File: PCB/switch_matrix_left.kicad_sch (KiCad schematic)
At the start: 80 parts, among them SW1 SW_Push, SW10 SW_Push, SW11 SW_Push, SW12 SW_Push, SW13 SW_Push, SW14 SW_Push, SW15 SW_Push, SW16 SW_Push, SW17 SW_Push, SW18 SW_Push, SW19 SW_Push, SW2 SW_Push, SW20 SW_Push, SW21 SW_Push, SW22 SW_Push, SW23 SW_Push, SW24 SW_Push, SW25 SW_Push, SW26 SW_Push, SW27 SW_Push, SW28 SW_Push, SW29 SW_Push, SW3 SW_Push, SW30 SW_Push, SW31 SW_Push, SW32 SW_Push, SW33 SW_Push, SW34 SW_Push, SW35 SW_Push, SW36 SW_Push, SW37 SW_Push, SW38 SW_Push, SW39 SW_Push, SW4 SW_Push, SW40 RotaryEncoder_Switch, SW5 SW_Push, SW6 SW_Push, SW7 SW_Push, SW8 SW_Push, SW9 SW_Push

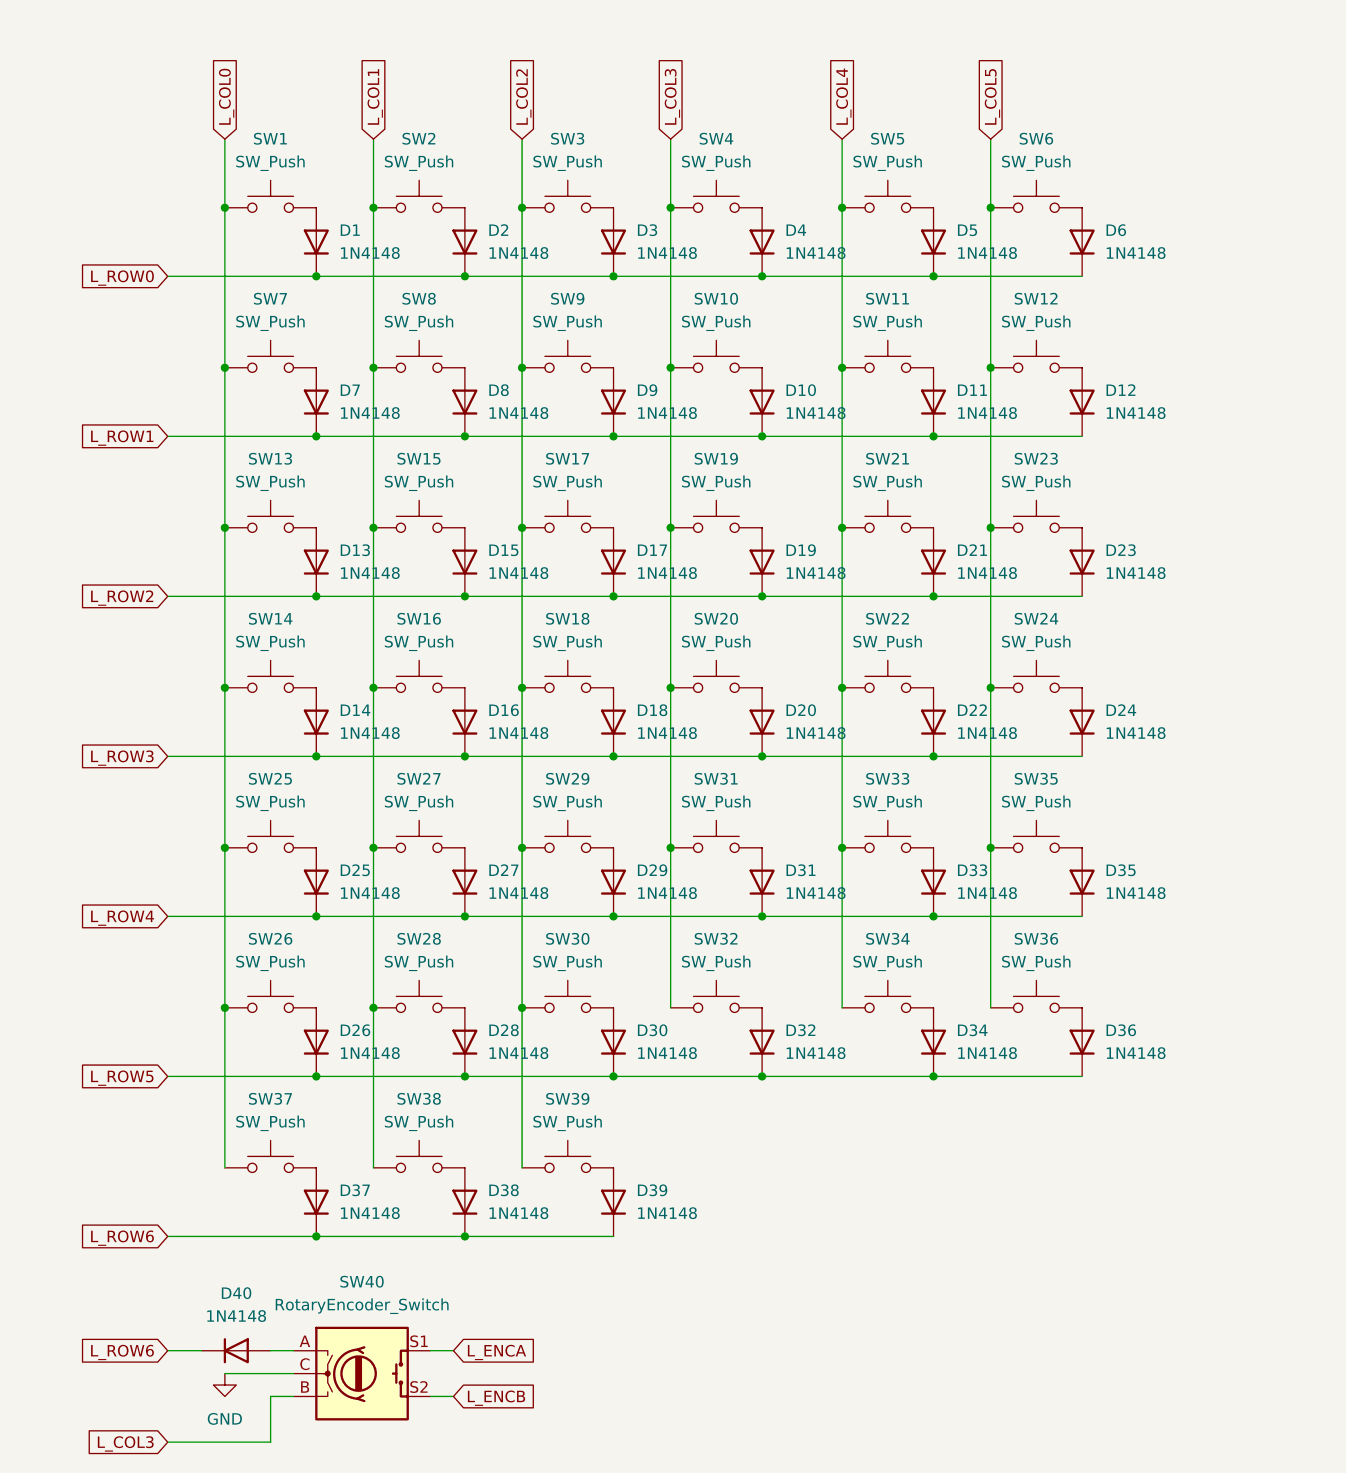
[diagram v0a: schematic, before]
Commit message: updated schematic
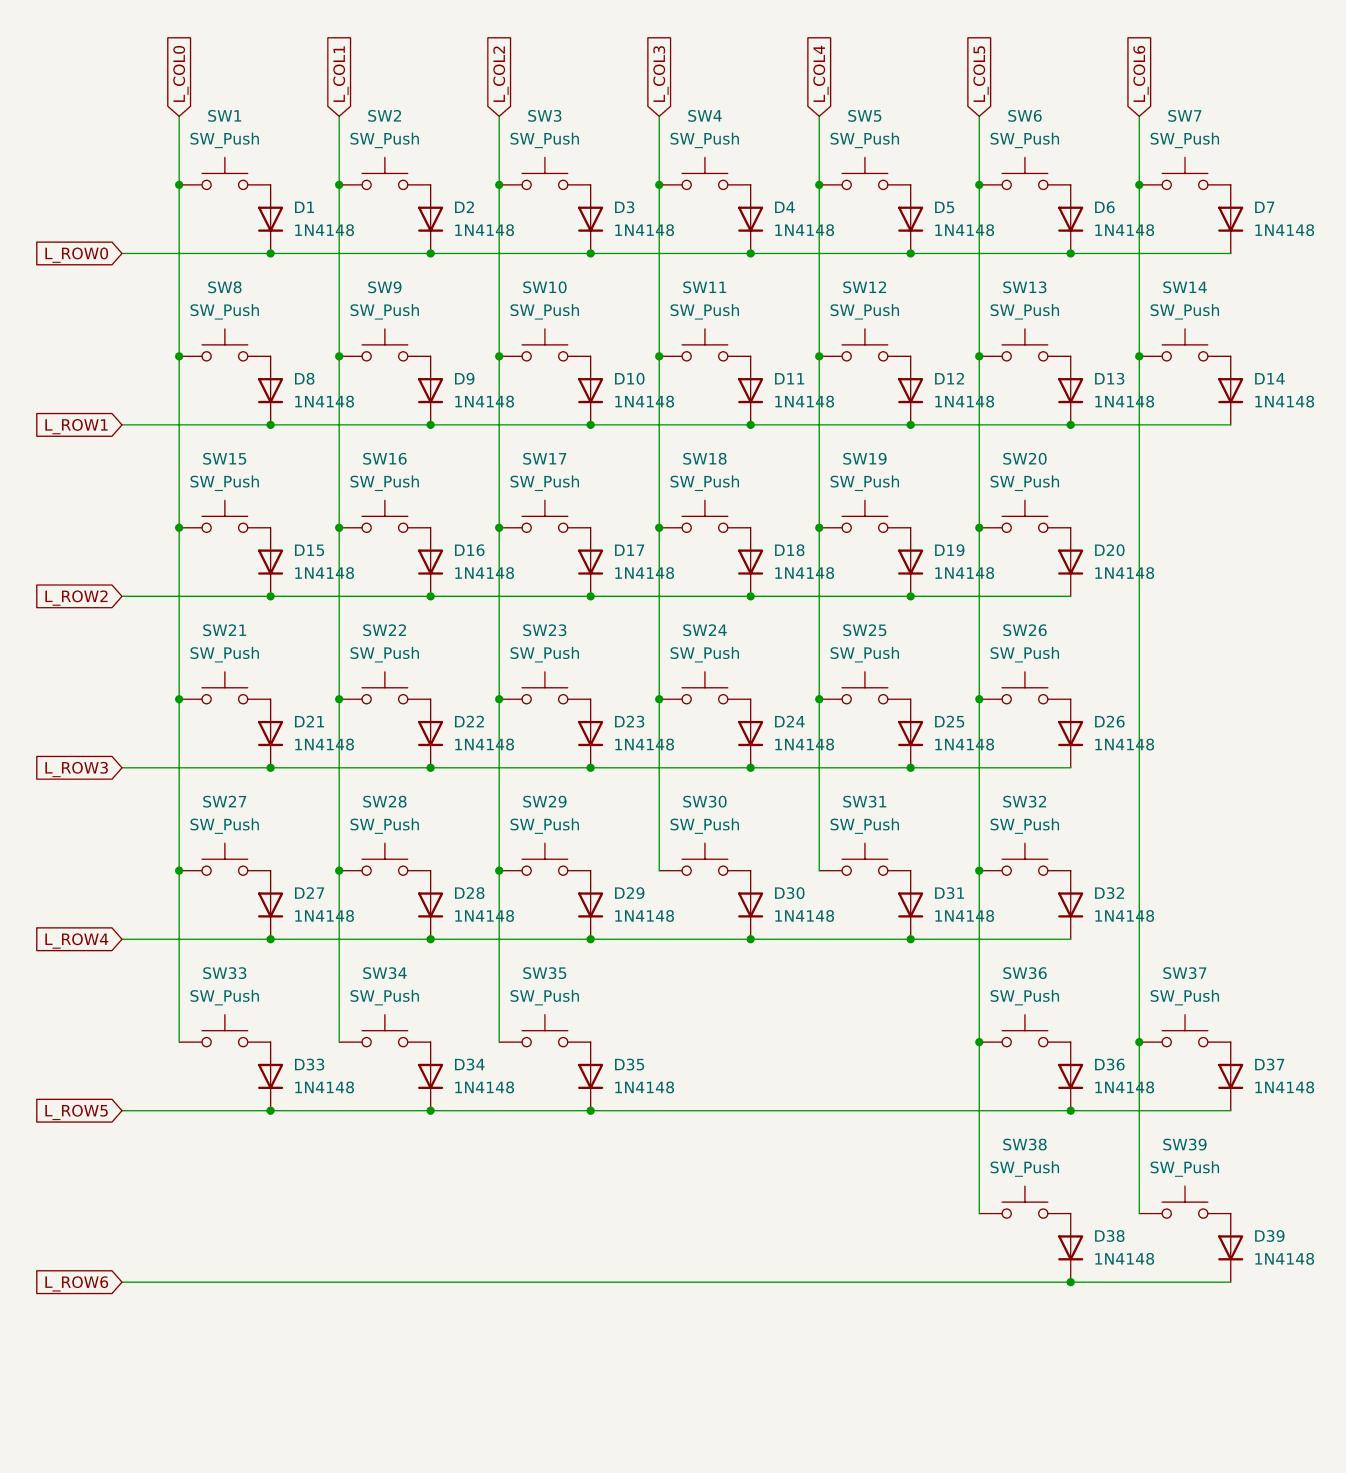
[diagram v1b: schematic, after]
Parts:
- removed D40: 1N4148, Diode_THT:D_DO-35_SOD27_P7.62mm_Horizontal, symbol Diode:1N4148
- removed SW40: RotaryEncoder_Switch, Rotary_Encoder:RotaryEncoder_Alps_EC11E-Switch_Vertical_H20mm, symbol Device:RotaryEncoder_Switch
- SW1, SW10, SW11, SW12, SW13, SW14, SW15, SW16, SW17, SW18, SW19, SW2, SW20, SW21, SW22, SW25, SW26, SW27, SW28, SW29, SW3, SW31, SW32, SW33, SW34, SW37, SW38, SW4, SW5, SW6, SW7, SW8, SW9: footprint Gateron_KS33_Hotswap:Gateron-KS33-Hotswap-1U -> (none)
- SW23, SW24, SW35, SW36: footprint Gateron_KS33_Hotswap:Gateron-KS33-Hotswap-1.25U -> (none)
- SW30, SW39: footprint Gateron_KS33_Hotswap:Gateron-KS33-Hotswap-2U -> (none)
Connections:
- net L_COL0: now also SW15.1, SW21.1, SW27.1, SW33.1, SW8.1; no longer SW13.1, SW14.1, SW25.1, SW26.1, SW37.1, SW7.1
- net L_COL1: now also SW22.1, SW34.1, SW9.1; no longer SW15.1, SW27.1, SW38.1, SW8.1
- net L_COL2: now also SW10.1, SW23.1, SW35.1; no longer SW18.1, SW30.1, SW39.1, SW9.1
- net L_COL3: now also SW11.1, SW18.1, SW24.1, SW30.1; no longer SW10.1, SW19.1, SW20.1, SW31.1, SW32.1
- net L_COL4: now also SW12.1, SW19.1, SW25.1, SW31.1; no longer SW11.1, SW21.1, SW22.1, SW33.1, SW34.1
- net L_COL5: now also SW13.1, SW20.1, SW26.1, SW32.1, SW38.1; no longer SW12.1, SW23.1, SW24.1, SW35.1
- net L_ROW0: now also D7.1 (K)
- net L_ROW1: now also D13.1 (K), D14.1 (K); no longer D7.1 (K)
- net L_ROW2: now also D16.1 (K), D18.1 (K), D20.1 (K); no longer D13.1 (K), D21.1 (K), D23.1 (K)
- net L_ROW3: now also D21.1 (K), D23.1 (K), D25.1 (K), D26.1 (K); no longer D14.1 (K), D16.1 (K), D18.1 (K), D20.1 (K)
- net L_ROW4: now also D28.1 (K), D30.1 (K), D32.1 (K); no longer D25.1 (K), D33.1 (K), D35.1 (K)
- net L_ROW5: now also D33.1 (K), D35.1 (K), D37.1 (K); no longer D26.1 (K), D28.1 (K), D30.1 (K), D32.1 (K)
- net L_ROW6: no longer D37.1 (K)
- new net L_COL6: SW14.1, SW37.1, SW39.1, SW7.1

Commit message: routed the switches and diodes
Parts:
- SW1, SW10, SW11, SW12, SW13, SW14, SW16, SW17, SW18, SW19, SW2, SW20, SW22, SW23, SW24, SW25, SW26, SW28, SW29, SW3, SW30, SW31, SW32, SW34, SW35, SW37, SW39, SW4, SW5, SW6, SW7, SW8, SW9: footprint (none) -> Gateron_KS33_Hotswap:Gateron-KS33-Hotswap-1U
- SW15, SW21, SW27, SW33: footprint (none) -> Gateron_KS33_Hotswap:Gateron-KS33-Hotswap-1.25U
- SW36, SW38: footprint (none) -> Gateron_KS33_Hotswap:Gateron-KS33-Hotswap-2U
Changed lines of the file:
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@@
 			)
 		)
-		(property "Footprint" ""
+		(property "Footprint" "Gateron_KS33_Hotswap:Gateron-KS33-Hotswap-1U"
 			(at 124.46 44.45 0)
 			(effects
@@
 			)
 		)
-		(property "Footprint" ""
+		(property "Footprint" "Gateron_KS33_Hotswap:Gateron-KS33-Hotswap-1U"
 			(at 88.9 82.55 0)
 			(effects
@@
 			)
 		)
-		(property "Footprint" ""
+		(property "Footprint" "Gateron_KS33_Hotswap:Gateron-KS33-Hotswap-1U"
 			(at 88.9 25.4 0)
 			(effects
@@
 			)
 		)
-		(property "Footprint" ""
+		(property "Footprint" "Gateron_KS33_Hotswap:Gateron-KS33-Hotswap-1U"
 			(at 142.24 25.4 0)
 			(effects
@@
 			)
 		)
-		(property "Footprint" ""
+		(property "Footprint" "Gateron_KS33_Hotswap:Gateron-KS33-Hotswap-1U"
 			(at 142.24 139.7 0)
 			(effects
@@
 			)
 		)
-		(property "Footprint" ""
+		(property "Footprint" "Gateron_KS33_Hotswap:Gateron-KS33-Hotswap-1U"
 			(at 106.68 25.4 0)
 			(effects
@@
 			)
 		)
-		(property "Footprint" ""
+		(property "Footprint" "Gateron_KS33_Hotswap:Gateron-KS33-Hotswap-1U"
 			(at 124.46 25.4 0)
 			(effects
@@
 			)
 		)
-		(property "Footprint" ""
+		(property "Footprint" "Gateron_KS33_Hotswap:Gateron-KS33-Hotswap-1U"
 			(at 71.12 44.45 0)
 			(effects
@@
 			)
 		)
-		(property "Footprint" ""
+		(property "Footprint" "Gateron_KS33_Hotswap:Gateron-KS33-Hotswap-1.25U"
 			(at 35.56 101.6 0)
 			(effects
@@
 			)
 		)
-		(property "Footprint" ""
+		(property "Footprint" "Gateron_KS33_Hotswap:Gateron-KS33-Hotswap-1U"
 			(at 53.34 101.6 0)
 			(effects
@@
 			)
 		)
-		(property "Footprint" ""
+		(property "Footprint" "Gateron_KS33_Hotswap:Gateron-KS33-Hotswap-1U"
 			(at 53.34 82.55 0)
 			(effects
@@
 			)
 		)
-		(property "Footprint" ""
+		(property "Footprint" "Gateron_KS33_Hotswap:Gateron-KS33-Hotswap-1U"
 			(at 142.24 44.45 0)
 			(effects
@@
 			)
 		)
-		(property "Footprint" ""
+		(property "Footprint" "Gateron_KS33_Hotswap:Gateron-KS33-Hotswap-1U"
 			(at 71.12 63.5 0)
 			(effects
@@
 			)
 		)
-		(property "Footprint" ""
+		(property "Footprint" "Gateron_KS33_Hotswap:Gateron-KS33-Hotswap-1U"
 			(at 71.12 120.65 0)
 			(effects
@@
 			)
 		)
-		(property "Footprint" ""
+		(property "Footprint" "Gateron_KS33_Hotswap:Gateron-KS33-Hotswap-1U"
 			(at 106.68 44.45 0)
 			(effects
@@
 			)
 		)
-		(property "Footprint" ""
+		(property "Footprint" "Gateron_KS33_Hotswap:Gateron-KS33-Hotswap-1U"
 			(at 88.9 63.5 0)
 			(effects
@@
 			)
 		)
-		(property "Footprint" ""
+		(property "Footprint" "Gateron_KS33_Hotswap:Gateron-KS33-Hotswap-1U"
 			(at 35.56 25.4 0)
 			(effects
@@
 			)
 		)
-		(property "Footprint" ""
+		(property "Footprint" "Gateron_KS33_Hotswap:Gateron-KS33-Hotswap-1U"
 			(at 88.9 44.45 0)
 			(effects
@@
 			)
 		)
-		(property "Footprint" ""
+		(property "Footprint" "Gateron_KS33_Hotswap:Gateron-KS33-Hotswap-2U"
 			(at 124.46 120.65 0)
 			(effects
@@
 			)
 		)
-		(property "Footprint" ""
+		(property "Footprint" "Gateron_KS33_Hotswap:Gateron-KS33-Hotswap-1U"
 			(at 124.46 63.5 0)
 			(effects
@@
 			)
 		)
-		(property "Footprint" ""
+		(property "Footprint" "Gateron_KS33_Hotswap:Gateron-KS33-Hotswap-1U"
 			(at 124.46 82.55 0)
 			(effects
@@
 			)
 		)
-		(property "Footprint" ""
+		(property "Footprint" "Gateron_KS33_Hotswap:Gateron-KS33-Hotswap-1U"
 			(at 124.46 101.6 0)
 			(effects
@@
 			)
 		)
-		(property "Footprint" ""
+		(property "Footprint" "Gateron_KS33_Hotswap:Gateron-KS33-Hotswap-1.25U"
 			(at 35.56 63.5 0)
 			(effects
@@
 			)
 		)
-		(property "Footprint" ""
+		(property "Footprint" "Gateron_KS33_Hotswap:Gateron-KS33-Hotswap-1U"
 			(at 142.24 120.65 0)
 			(effects
@@
 			)
 		)
-		(property "Footprint" ""
+		(property "Footprint" "Gateron_KS33_Hotswap:Gateron-KS33-Hotswap-1U"
 			(at 53.34 63.5 0)
 			(effects
@@
 			)
 		)
-		(property "Footprint" ""
+		(property "Footprint" "Gateron_KS33_Hotswap:Gateron-KS33-Hotswap-1.25U"
 			(at 35.56 82.55 0)
 			(effects
@@
 			)
 		)
-		(property "Footprint" ""
+		(property "Footprint" "Gateron_KS33_Hotswap:Gateron-KS33-Hotswap-1.25U"
 			(at 35.56 120.65 0)
 			(effects
@@
 			)
 		)
-		(property "Footprint" ""
+		(property "Footprint" "Gateron_KS33_Hotswap:Gateron-KS33-Hotswap-1U"
 			(at 106.68 101.6 0)
 			(effects
@@
 			)
 		)
-		(property "Footprint" ""
+		(property "Footprint" "Gateron_KS33_Hotswap:Gateron-KS33-Hotswap-1U"
 			(at 71.12 101.6 0)
 			(effects
@@
 			)
 		)
-		(property "Footprint" ""
+		(property "Footprint" "Gateron_KS33_Hotswap:Gateron-KS33-Hotswap-2U"
 			(at 124.46 139.7 0)
 			(effects
@@
 			)
 		)
-		(property "Footprint" ""
+		(property "Footprint" "Gateron_KS33_Hotswap:Gateron-KS33-Hotswap-1U"
 			(at 53.34 120.65 0)
 			(effects
@@
 			)
 		)
-		(property "Footprint" ""
+		(property "Footprint" "Gateron_KS33_Hotswap:Gateron-KS33-Hotswap-1U"
 			(at 106.68 63.5 0)
 			(effects
@@
 			)
 		)
-		(property "Footprint" ""
+		(property "Footprint" "Gateron_KS33_Hotswap:Gateron-KS33-Hotswap-1U"
 			(at 71.12 82.55 0)
 			(effects
@@
 			)
 		)
-		(property "Footprint" ""
+		(property "Footprint" "Gateron_KS33_Hotswap:Gateron-KS33-Hotswap-1U"
 			(at 88.9 101.6 0)
 			(effects
@@
 			)
 		)
-		(property "Footprint" ""
+		(property "Footprint" "Gateron_KS33_Hotswap:Gateron-KS33-Hotswap-1U"
 			(at 53.34 25.4 0)
 			(effects
@@
 			)
 		)
-		(property "Footprint" ""
+		(property "Footprint" "Gateron_KS33_Hotswap:Gateron-KS33-Hotswap-1U"
 			(at 35.56 44.45 0)
 			(effects
@@
 			)
 		)
-		(property "Footprint" ""
+		(property "Footprint" "Gateron_KS33_Hotswap:Gateron-KS33-Hotswap-1U"
 			(at 53.34 44.45 0)
 			(effects
@@
 			)
 		)
-		(property "Footprint" ""
+		(property "Footprint" "Gateron_KS33_Hotswap:Gateron-KS33-Hotswap-1U"
 			(at 106.68 82.55 0)
 			(effects
@@
 			)
 		)
-		(property "Footprint" ""
+		(property "Footprint" "Gateron_KS33_Hotswap:Gateron-KS33-Hotswap-1U"
 			(at 71.12 25.4 0)
 			(effects
